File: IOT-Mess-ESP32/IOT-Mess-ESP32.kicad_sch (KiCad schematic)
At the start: 35 parts, among them J1 Conn_01x05_Pin, J2 SuperMini_ESP32-H2, J3 Conn_01x05_Pin, J5 Conn_01x24_Pin, J6 USB_C_Receptacle_USB2.0_16P, SW1 RotaryEncoder, SW10 SW_Push, SW11 SW_Push, U1 ESP-12F, U3 ESP32-S3-WROOM-1, U4 ME6211C33M5, U5 ESP32-C3-WROOM-02

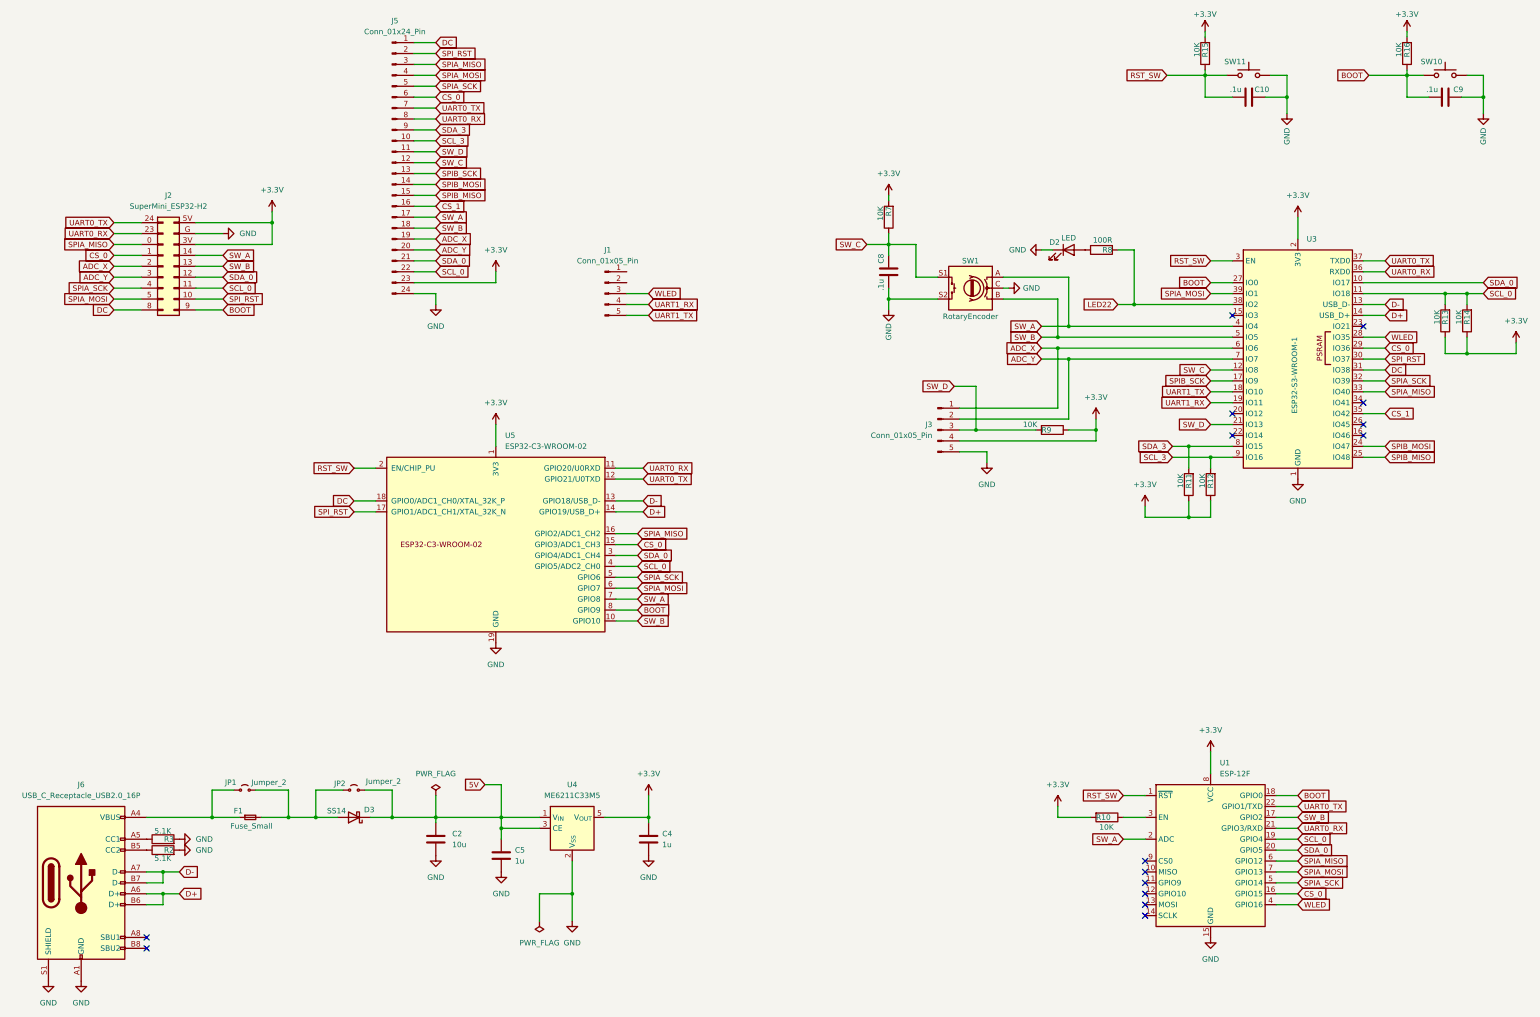
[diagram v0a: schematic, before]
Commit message: did some works.
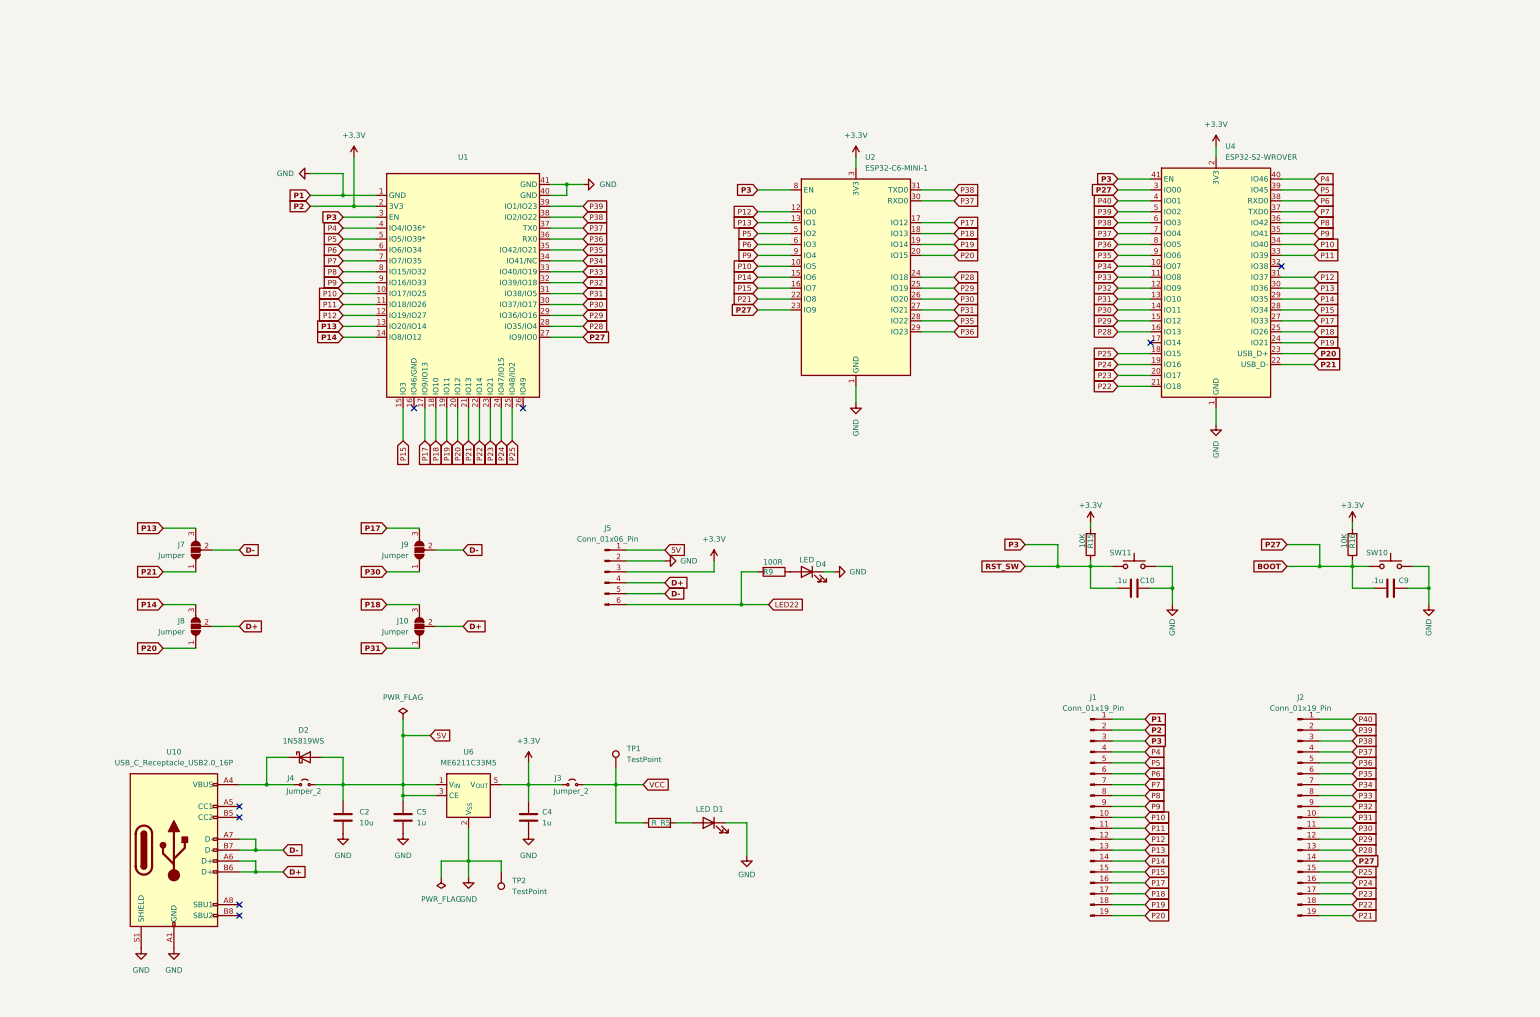
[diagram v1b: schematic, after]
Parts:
- removed C8: .1u, Capacitor_SMD:C_0603_1608Metric, symbol Device:C
- removed D2: LED, LED_SMD:LED_0603_1608Metric, symbol Device:LED
- removed D3: SS14, Diode_SMD:D_SMA, symbol Diode:SS14
- removed F1: Fuse_Small, symbol Device:Fuse_Small
- removed J1: Conn_01x05_Pin, Connector_PinHeader_2.54mm:PinHeader_1x05_P2.54mm_Vertical, symbol Connector:Conn_01x05_Pin
- removed J2: SuperMini_ESP32-H2, symbol IOT-Mess:SuperMini_ESP32-H2
- removed J3: Conn_01x05_Pin, Connector_PinSocket_2.54mm:PinSocket_1x05_P2.54mm_Vertical, symbol Connector:Conn_01x05_Pin
- removed J5: Conn_01x24_Pin, Connector_PinHeader_2.54mm:PinHeader_1x24_P2.54mm_Vertical, symbol Connector:Conn_01x24_Pin
- removed JP1, JP2: Jumper_2, Jumper:SolderJumper-2_P1.3mm_Open_Pad1.0x1.5mm, symbol Jumper:Jumper_2_Small_Open
- removed R10, R11, R12, R13, R14, R7: 10K, Resistor_SMD:R_0603_1608Metric, symbol Device:R
- removed R2, R3: 5.1K, Resistor_SMD:R_0603_1608Metric, symbol Device:R
- removed R8: 100R, Resistor_SMD:R_0603_1608Metric, symbol Device:R
- removed SW1: RotaryEncoder, IOT-Mess-Footprints:RotaryEncoder_EC11_SMD, symbol Device:RotaryEncoder_Switch
- removed U1: ESP-12F, RF_Module:ESP-12E, symbol RF_Module:ESP-12F
- removed U3: ESP32-S3-WROOM-1, RF_Module:ESP32-S3-WROOM-1, symbol RF_Module:ESP32-S3-WROOM-1
- removed U4: ME6211C33M5, Package_TO_SOT_SMD:SOT-23-5, symbol Regulator_Linear:ME6211C33M5
- removed U5: ESP32-C3-WROOM-02, RF_Module:ESP32-C3-WROOM-02, symbol Espressif:ESP32-C3-WROOM-02
- added D1, D4: LED, LED_SMD:LED_0603_1608Metric, symbol Device:LED
- added D2: 1N5819WS, Diode_SMD:D_SOD-323, symbol Diode:1N5819WS
- added J1, J2: Conn_01x19_Pin, Connector_PinHeader_2.54mm:PinHeader_1x19_P2.54mm_Vertical, symbol Connector:Conn_01x19_Pin
- added J10, J7, J8, J9: Jumper, IOT-Mess-Footprints:Jumper-3_P1.3mm_Open_RoundedPad1.0x1.5mm, symbol Jumper:SolderJumper_3_Open
- added J3, J4: Jumper_2, IOT-Mess-Footprints:Jumpper-triangle, symbol Jumper:Jumper_2_Small_Open
- added J5: Conn_01x06_Pin, Connector_PinHeader_2.54mm:PinHeader_1x06_P2.54mm_Vertical, symbol Connector:Conn_01x06_Pin
- added R5: R, Resistor_SMD:R_0603_1608Metric, symbol Device:R
- added TP1, TP2: TestPoint, symbol Connector:TestPoint
- added U1: ~, Espressif:ESP32-S3-WROOM-1, symbol IOT-Mess:ESP32-S3
- added U2: ESP32-C6-MINI-1, RF_Module:ESP32-C6-MINI-1, symbol RF_Module:ESP32-C6-MINI-1
- added U4: ESP32-S2-WROVER, RF_Module:ESP32-S2-WROVER, symbol RF_Module:ESP32-S2-WROVER
- added U6: ME6211C33M5, Package_TO_SOT_SMD:SOT-23-5, symbol Regulator_Linear:ME6211C33M5
- R9: value 10K -> 100R
- renumbered J6 to U10
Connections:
- net SW_D is gone; now on net LED22: R9.2
- net +3.3V: now also J1.2 (Pin_2), J3.1 (A), J5.3 (Pin_3), U1.2 (3V3), U2.3 (3V3), U4.2 (3V3), U6.5 (V_{OUT}); no longer R9.1
- net 5V: now also D2.2 (A), J4.2 (B), J5.1 (Pin_1), U6.1 (V_{IN}), U6.3 (CE)
- net BOOT: now also J2.14 (Pin_14), U1.27 (IO9/IO0), U2.23 (IO9), U4.3 (IO00)
- net D+: now also J10.2 (C), J5.4 (Pin_4), J8.2 (C)
- net D-: now also J5.5 (Pin_5), J7.2 (C), J9.2 (C)
- net GND: now also D1.1 (K), D4.1 (K), J1.1 (Pin_1), J5.2 (Pin_2), TP2.1, U1.1 (GND), U1.40 (GND), U1.41 (GND), U2.1 (GND), U2.11 (GND), U2.14 (GND), U2.2 (GND), U2.36 (GND), U2.37 (GND), U2.38 (GND), U2.39 (GND), U2.40 (GND), U2.41 (GND), U2.42 (GND), U2.43 (GND), U2.44 (GND), U2.45 (GND), U2.46 (GND), U2.47 (GND), U2.48 (GND), U2.49 (GND), U2.50 (GND), U2.51 (GND), U2.52 (GND), U2.53 (GND), U4.1 (GND), U4.26 (GND), U4.42 (GND), U4.43 (GND), U6.2 (V_{SS})
- net LED22: now also J5.6 (Pin_6)
- net at U10.A4 (VBUS), U10.A9 (VBUS), U10.B4 (VBUS)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: now also D2.1 (K), J4.1 (A)
- net RST_SW renamed P3
- net P3: now also J1.3 (Pin_3), U1.3 (EN), U2.8 (EN), U4.41 (EN)
- new net: D4.2 (A), R9.1
- new net: D1.2 (A), R5.2
- new net P10: J1.10 (Pin_10), U1.10 (IO17/IO25), U2.10 (IO5), U4.34 (IO40)
- new net P11: J1.11 (Pin_11), U1.11 (IO18/IO26), U4.33 (IO39)
- new net P12: J1.12 (Pin_12), U1.12 (IO19/IO27), U2.12 (IO0), U4.31 (IO37)
- new net P13: J1.13 (Pin_13), J7.3 (B), U1.13 (IO20/IO14), U2.13 (IO1), U4.30 (IO36)
- new net P14: J1.14 (Pin_14), J8.3 (B), U1.14 (IO8/IO12), U2.15 (IO6), U4.29 (IO35)
- new net P15: J1.15 (Pin_15), U1.15 (IO3), U2.16 (IO7), U4.28 (IO34)
- new net P17: J1.16 (Pin_16), J9.3 (B), U1.17 (IO9/IO13), U2.17 (IO12), U4.27 (IO33)
- new net P18: J1.17 (Pin_17), J10.3 (B), U1.18 (IO10), U2.18 (IO13), U4.25 (IO26)
- new net P19: J1.18 (Pin_18), U1.19 (IO11), U2.19 (IO14), U4.24 (IO21)
- new net P20: J1.19 (Pin_19), J8.1 (A), U1.20 (IO12), U2.20 (IO15), U4.23 (USB_D+)
- new net P21: J2.19 (Pin_19), J7.1 (A), U1.21 (IO13), U2.22 (IO8), U4.22 (USB_D-)
- new net P22: J2.18 (Pin_18), U1.22 (IO14), U4.21 (IO18)
- new net P23: J2.17 (Pin_17), U1.23 (IO21), U4.20 (IO17)
- new net P24: J2.16 (Pin_16), U1.24 (IO47/IO15), U4.19 (IO16)
- new net P25: J2.15 (Pin_15), U1.25 (IO48/IO2), U4.18 (IO15)
- new net P28: J2.13 (Pin_13), U1.28 (IO35/IO4), U2.24 (IO18), U4.16 (IO13)
- new net P29: J2.12 (Pin_12), U1.29 (IO36/IO16), U2.25 (IO19), U4.15 (IO12)
- new net P30: J2.11 (Pin_11), J9.1 (A), U1.30 (IO37/IO17), U2.26 (IO20), U4.14 (IO11)
- new net P31: J10.1 (A), J2.10 (Pin_10), U1.31 (IO38/IO5), U2.27 (IO21), U4.13 (IO10)
- new net P32: J2.9 (Pin_9), U1.32 (IO39/IO18), U4.12 (IO09)
- new net P33: J2.8 (Pin_8), U1.33 (IO40/IO19), U4.11 (IO08)
- new net P34: J2.7 (Pin_7), U1.34 (IO41/NC), U4.10 (IO07)
- new net P35: J2.6 (Pin_6), U1.35 (IO42/IO21), U2.28 (IO22), U4.9 (IO06)
- new net P36: J2.5 (Pin_5), U1.36 (RX0), U2.29 (IO23), U4.8 (IO05)
- new net P37: J2.4 (Pin_4), U1.37 (TX0), U2.30 (RXD0), U4.7 (IO04)
- new net P38: J2.3 (Pin_3), U1.38 (IO2/IO22), U2.31 (TXD0), U4.6 (IO03)
- new net P39: J2.2 (Pin_2), U1.39 (IO1/IO23), U4.5 (IO02)
- new net P4: J1.4 (Pin_4), U1.4 (IO4/IO36*), U4.40 (IO46)
- new net P40: J2.1 (Pin_1), U4.4 (IO01)
- new net P5: J1.5 (Pin_5), U1.5 (IO5/IO39*), U2.5 (IO2), U4.39 (IO45)
- new net P6: J1.6 (Pin_6), U1.6 (IO6/IO34), U2.6 (IO3), U4.38 (RXD0)
- new net P7: J1.7 (Pin_7), U1.7 (IO7/IO35), U4.37 (TXD0)
- new net P8: J1.8 (Pin_8), U1.8 (IO15/IO32), U4.36 (IO42)
- new net P9: J1.9 (Pin_9), U1.9 (IO16/IO33), U2.9 (IO4), U4.35 (IO41)
- new net VCC: J3.2 (B), R5.1, TP1.1
- no-connect marks 15 -> 8
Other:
- moved on the sheet: C10, C2, C4, C5, C9, R15, R16, SW10, SW11, U10
